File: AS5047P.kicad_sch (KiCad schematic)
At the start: 3 parts, among them U6 AS5047P-ATSM

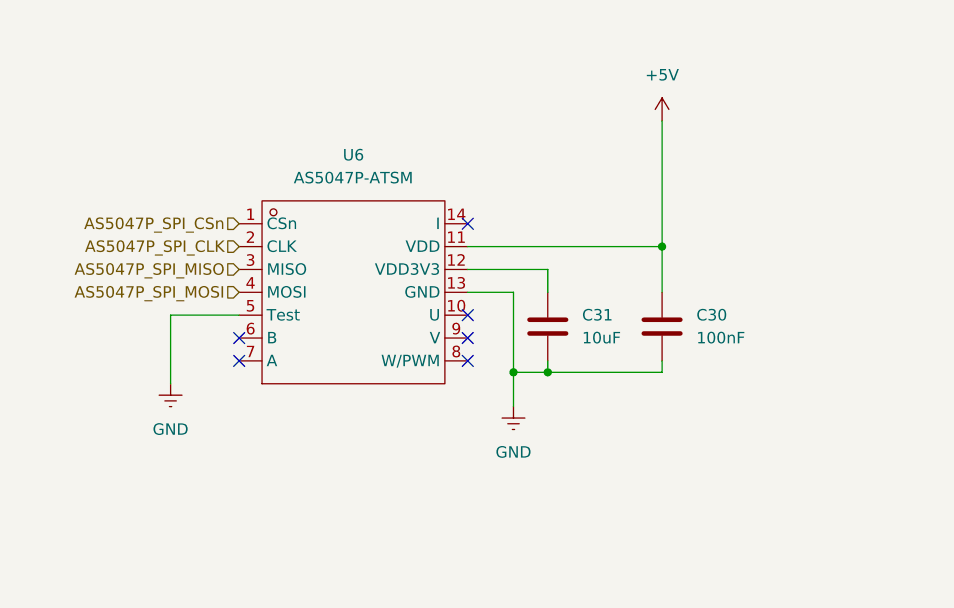
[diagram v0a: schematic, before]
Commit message: change components
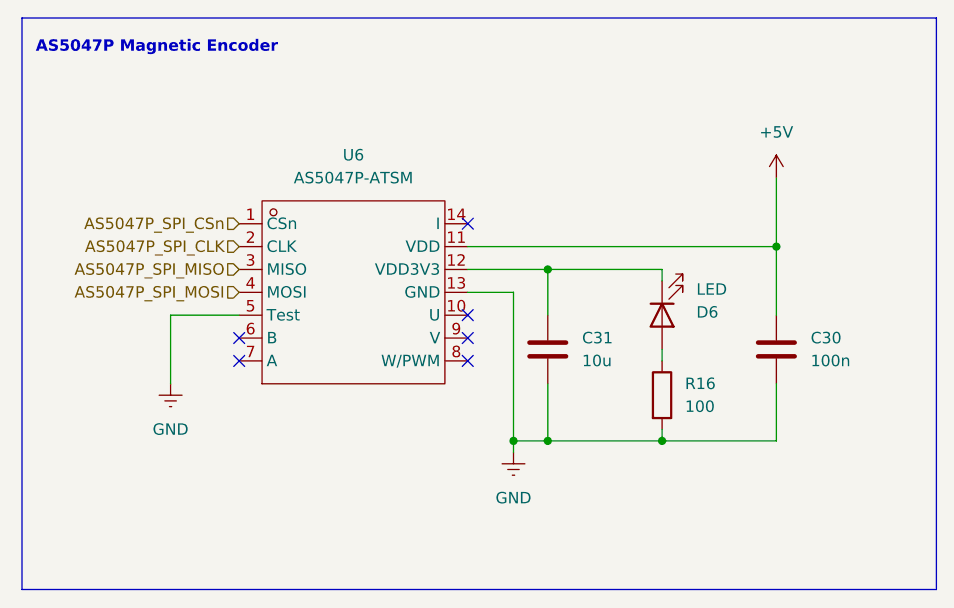
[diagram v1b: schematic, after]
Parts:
- added D6: LED, symbol Device:LED
- added R16: 100, PCM_Resistor_SMD_AKL:R_0402_1005Metric, symbol Device:R
- C30: value 100nF -> 100n; footprint (none) -> Capacitor_SMD:C_0402_1005Metric
- C31: value 10uF -> 10u; footprint (none) -> Capacitor_SMD:C_0402_1005Metric
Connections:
- net GND: now also R16.2
- net at C31.2, U6.12 (VDD3V3): now also D6.1 (K)
- new net: D6.2 (A), R16.1
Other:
- note added: "AS5047P Magnetic Encoder"
- moved on the sheet: C30, C31

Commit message: update sch
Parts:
- D6: footprint (none) -> LED_SMD:LED_0603_1608Metric
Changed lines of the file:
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@@
 			)
 		)
-		(property "Footprint" ""
+		(property "Footprint" "LED_SMD:LED_0603_1608Metric"
 			(at 172.72 96.52 0)
 			(effects
